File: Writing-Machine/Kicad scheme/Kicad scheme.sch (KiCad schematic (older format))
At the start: 1 part

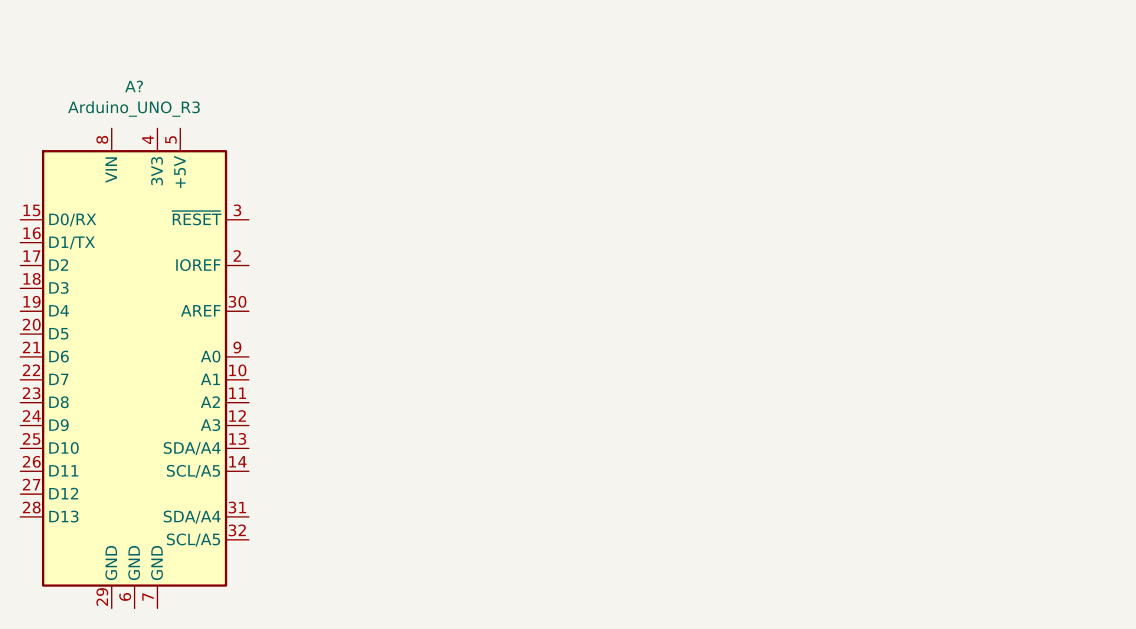
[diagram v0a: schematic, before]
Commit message: Add some work
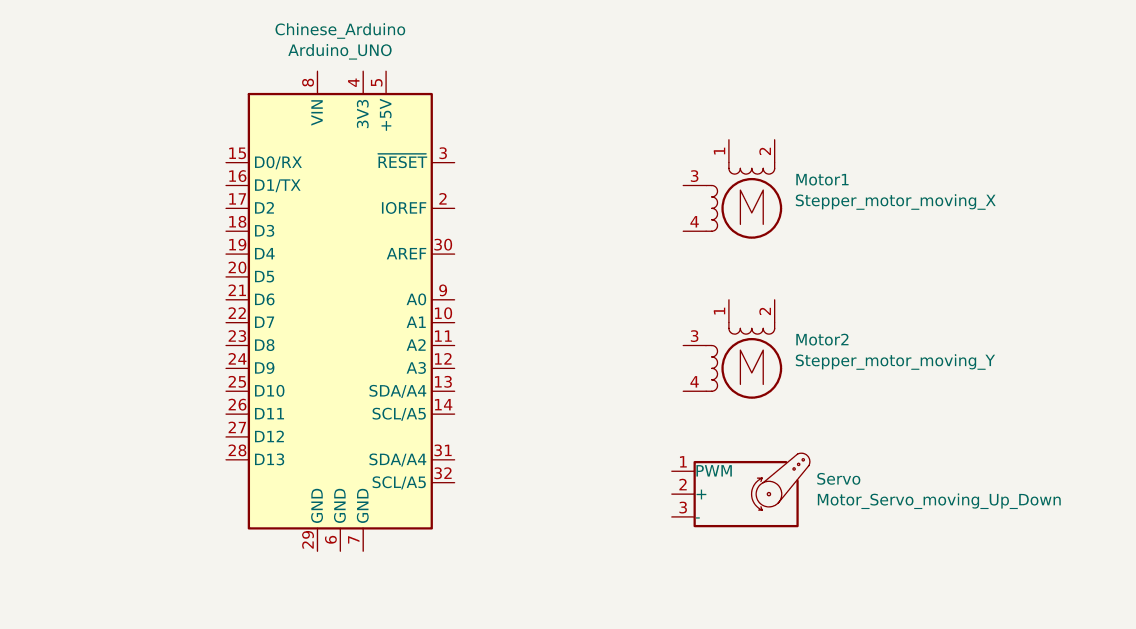
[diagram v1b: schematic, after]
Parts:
- added Motor1: Stepper_motor_moving_X, symbol Motor:Stepper_Motor_bipolar
- added Motor2: Stepper_motor_moving_Y, symbol Motor:Stepper_Motor_bipolar
- added Servo: Motor_Servo_moving_Up_Down, symbol Motor:Motor_Servo
- Chinese_Arduino: renamed from A?; value Arduino_UNO_R3 -> Arduino_UNO
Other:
- moved on the sheet: Chinese_Arduino
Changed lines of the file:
@@
 $EndDescr
 $Comp
-L MCU_Module:Arduino_UNO_R3 A?
+L MCU_Module:Arduino_UNO_R3 Chinese_Arduino
 U 1 1 5FDB88D6
-P 2950 3750
-F 0 "A?" H 2950 4931 50  0000 C CNN
-F 1 "Arduino_UNO_R3" H 2950 4840 50  0000 C CNN
-F 2 "Module:Arduino_UNO_R3" H 2950 3750 50  0001 C CIN
-F 3 "https://www.arduino.cc/en/Main/arduinoBoardUno" H 2950 3750 50  0001 C CNN
-	1    2950 3750
+P 3850 3500
+F 0 "Chinese_Arduino" H 3850 4681 50  0000 C CNN
+F 1 "Arduino_UNO" H 3850 4590 50  0000 C CNN
+F 2 "Module:Arduino_UNO_R3" H 3850 3500 50  0001 C CIN
+F 3 "https://www.arduino.cc/en/Main/arduinoBoardUno" H 3850 3500 50  0001 C CNN
+	1    3850 3500
 	1    0    0    -1
 $EndComp
+$Comp
+L Motor:Stepper_Motor_bipolar Motor1
+U 1 1 5FF2BB4E
+P 5650 3100
+F 0 "Motor1" H 5838 3224 50  0000 L CNN
+F 1 "Stepper_motor_moving_X" H 5838 3133 50  0000 L CNN
+F 2 "" H 5660 3090 50  0001 C CNN
+F 3 "http://www.infineon.com/dgdl/Application-Note-TLE8110EE_driving_UniPolarStepperMotor_V1.1.pdf?fileId=db3a30431be39b97011be5d0aa0a00b0" H 5660 3090 50  0001 C CNN
+	1    5650 3100
+	1    0    0    -1
+$EndComp
+$Comp
+L Motor:Stepper_Motor_bipolar Motor2
+U 1 1 5FF2EFA1
+P 5650 3800
+F 0 "Motor2" H 5838 3924 50  0000 L CNN
+F 1 "Stepper_motor_moving_Y" H 5838 3833 50  0000 L CNN
+F 2 "" H 5660 3790 50  0001 C CNN
+F 3 "http://www.infineon.com/dgdl/Application-Note-TLE8110EE_driving_UniPolarStepperMotor_V1.1.pdf?fileId=db3a30431be39b97011be5d0aa0a00b0" H 5660 3790 50  0001 C CNN
+	1    5650 3800
+	1    0    0    -1
+$EndComp
+$Comp
+L Motor:Motor_Servo Servo
+U 1 1 5FF389CD
+P 5600 4350
+F 0 "Servo" H 5932 4415 50  0000 L CNN
+F 1 "Motor_Servo_moving_Up_Down" H 5932 4324 50  0000 L CNN
+F 2 "" H 5600 4160 50  0001 C CNN
+F 3 "http://forums.parallax.com/uploads/attachments/46831/74481.png" H 5600 4160 50  0001 C CNN
+	1    5600 4350
+	1    0    0    -1
+$EndComp

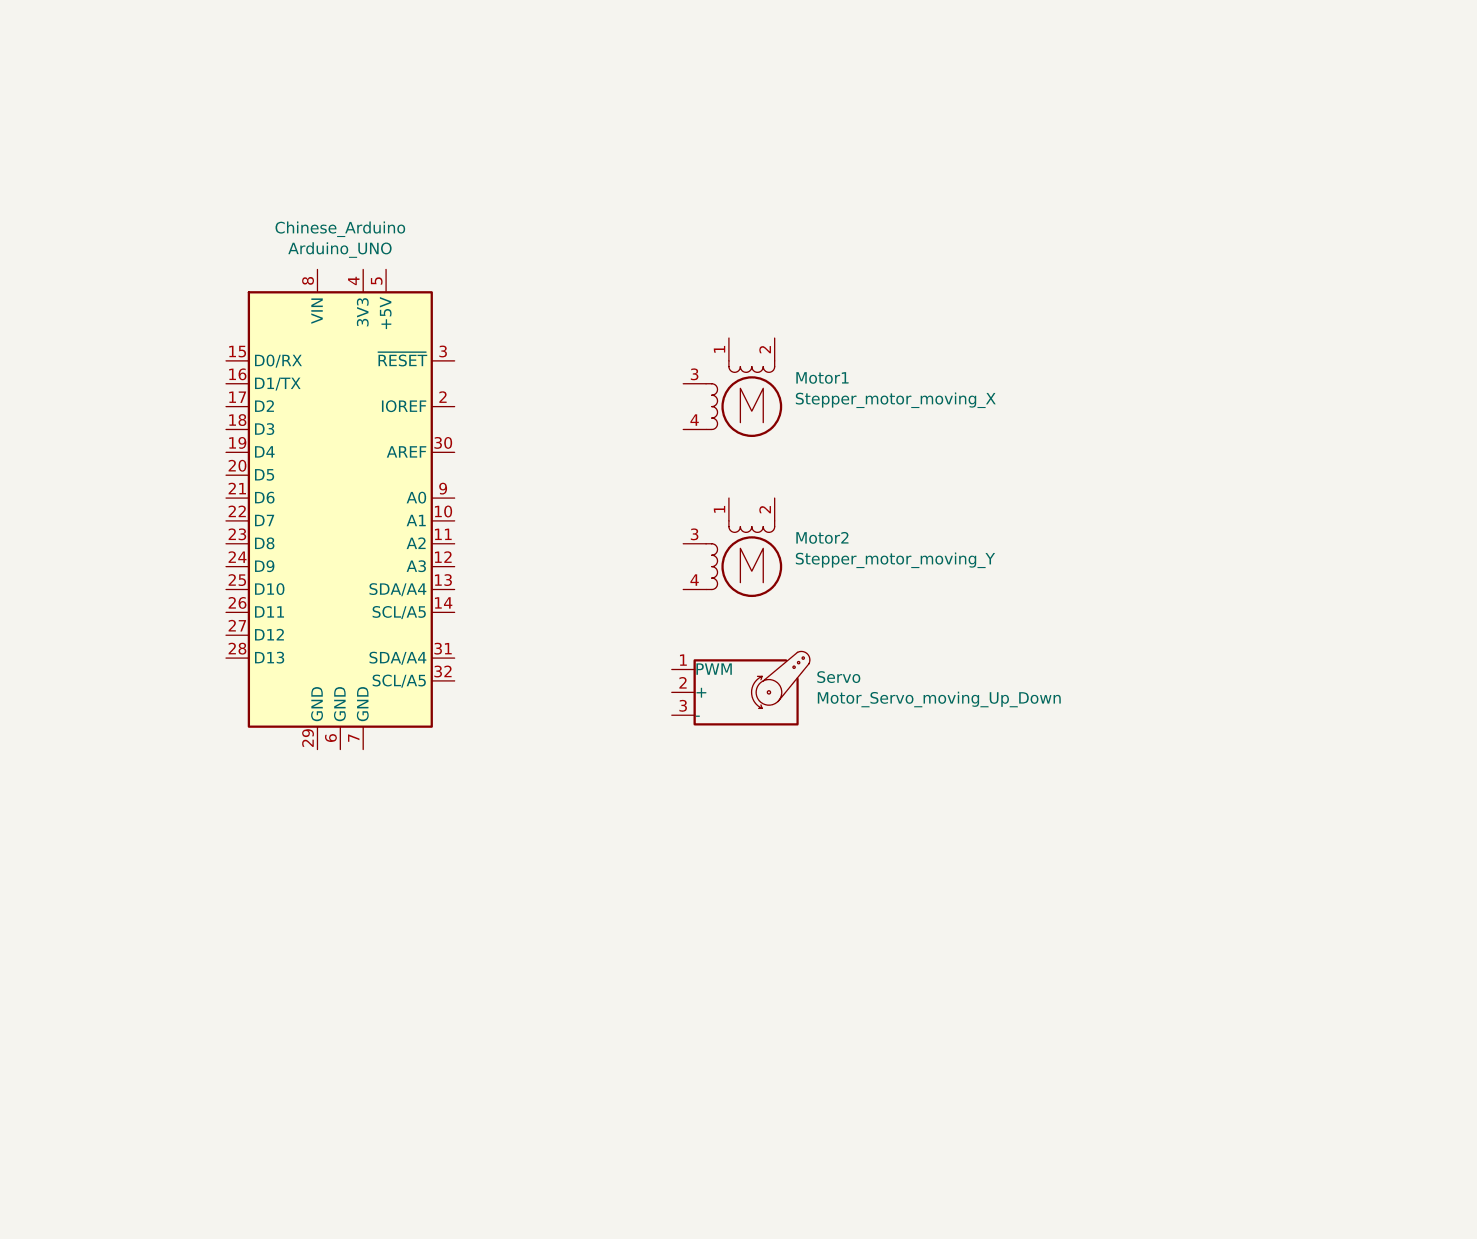
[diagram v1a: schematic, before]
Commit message: Add some night work
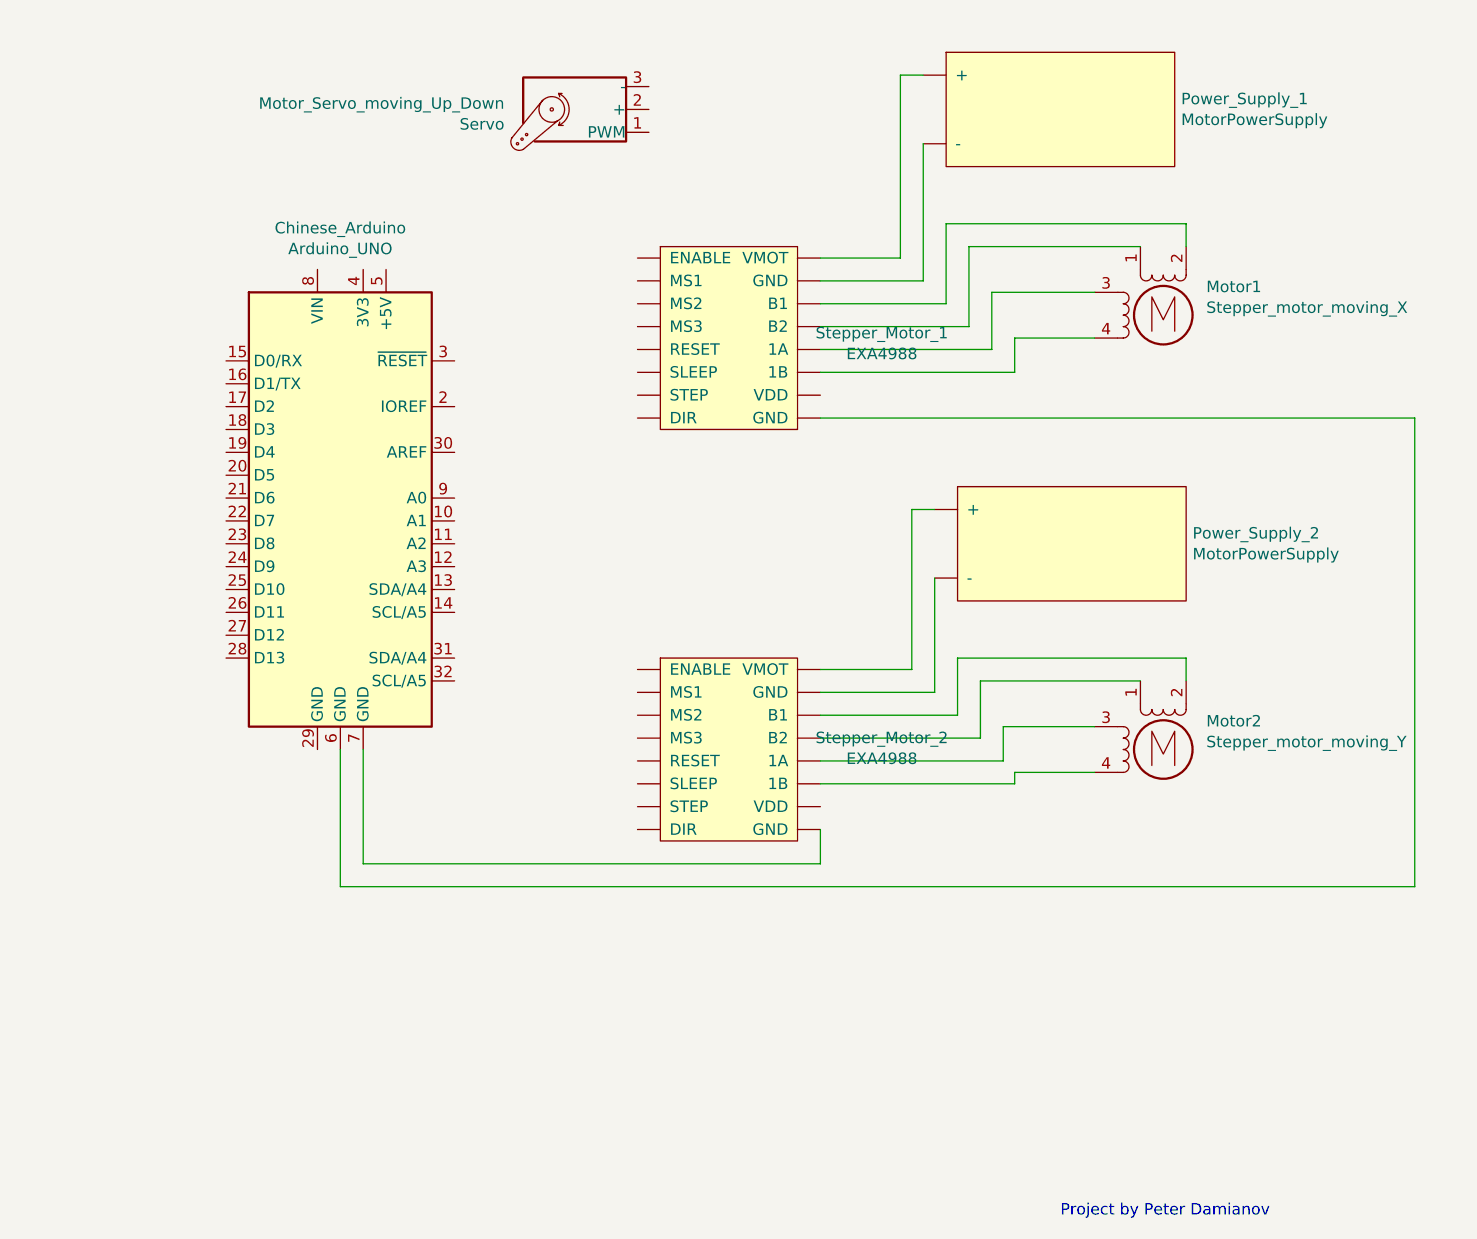
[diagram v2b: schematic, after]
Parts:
- added Power_Supply_1, Power_Supply_2: MotorPowerSupply, symbol Test:MotorPowerSupply
- added Stepper_Motor_1, Stepper_Motor_2: EXA4988, symbol Test:EXA4988
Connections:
- net at Chinese_Arduino.6 (GND): now also Stepper_Motor_1.~ (VMOT)
- net at Chinese_Arduino.7 (GND): now also Stepper_Motor_2.~ (VMOT)
- net at Motor1.1: now also Stepper_Motor_1.~ (VMOT)
- net at Motor1.2 (-): now also Stepper_Motor_1.~ (VMOT)
- net at Motor1.3: now also Stepper_Motor_1.~ (VMOT)
- net at Motor1.4: now also Stepper_Motor_1.~ (VMOT)
- net at Motor2.1: now also Stepper_Motor_2.~ (VMOT)
- net at Motor2.2 (-): now also Stepper_Motor_2.~ (VMOT)
- net at Motor2.3: now also Stepper_Motor_2.~ (VMOT)
- net at Motor2.4: now also Stepper_Motor_2.~ (VMOT)
- new net: Power_Supply_1.~ (-), Stepper_Motor_1.~ (VMOT) (x2)
- new net: Power_Supply_2.~ (-), Stepper_Motor_2.~ (VMOT) (x2)
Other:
- note added: "Project by Peter Damianov"
- moved on the sheet: Motor1, Motor2, Servo
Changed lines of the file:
@@
 L Motor:Stepper_Motor_bipolar Motor1
 U 1 1 5FF2BB4E
-P 5650 3100
-F 0 "Motor1" H 5838 3224 50  0000 L CNN
-F 1 "Stepper_motor_moving_X" H 5838 3133 50  0000 L CNN
-F 2 "" H 5660 3090 50  0001 C CNN
-F 3 "http://www.infineon.com/dgdl/Application-Note-TLE8110EE_driving_UniPolarStepperMotor_V1.1.pdf?fileId=db3a30431be39b97011be5d0aa0a00b0" H 5660 3090 50  0001 C CNN
-	1    5650 3100
+P 7450 2700
+F 0 "Motor1" H 7638 2824 50  0000 L CNN
+F 1 "Stepper_motor_moving_X" H 7638 2733 50  0000 L CNN
+F 2 "" H 7460 2690 50  0001 C CNN
+F 3 "http://www.infineon.com/dgdl/Application-Note-TLE8110EE_driving_UniPolarStepperMotor_V1.1.pdf?fileId=db3a30431be39b97011be5d0aa0a00b0" H 7460 2690 50  0001 C CNN
+	1    7450 2700
 	1    0    0    -1
 $EndComp
@@
 L Motor:Stepper_Motor_bipolar Motor2
 U 1 1 5FF2EFA1
-P 5650 3800
-F 0 "Motor2" H 5838 3924 50  0000 L CNN
-F 1 "Stepper_motor_moving_Y" H 5838 3833 50  0000 L CNN
-F 2 "" H 5660 3790 50  0001 C CNN
-F 3 "http://www.infineon.com/dgdl/Application-Note-TLE8110EE_driving_UniPolarStepperMotor_V1.1.pdf?fileId=db3a30431be39b97011be5d0aa0a00b0" H 5660 3790 50  0001 C CNN
-	1    5650 3800
+P 7450 4600
+F 0 "Motor2" H 7638 4724 50  0000 L CNN
+F 1 "Stepper_motor_moving_Y" H 7638 4633 50  0000 L CNN
+F 2 "" H 7460 4590 50  0001 C CNN
+F 3 "http://www.infineon.com/dgdl/Application-Note-TLE8110EE_driving_UniPolarStepperMotor_V1.1.pdf?fileId=db3a30431be39b97011be5d0aa0a00b0" H 7460 4590 50  0001 C CNN
+	1    7450 4600
 	1    0    0    -1
 $EndComp
@@
 L Motor:Motor_Servo Servo
 U 1 1 5FF389CD
-P 5600 4350
-F 0 "Servo" H 5932 4415 50  0000 L CNN
-F 1 "Motor_Servo_moving_Up_Down" H 5932 4324 50  0000 L CNN
-F 2 "" H 5600 4160 50  0001 C CNN
-F 3 "http://forums.parallax.com/uploads/attachments/46831/74481.png" H 5600 4160 50  0001 C CNN
-	1    5600 4350
+P 4900 1800
+F 0 "Servo" H 5232 1865 50  0000 L CNN
+F 1 "Motor_Servo_moving_Up_Down" H 5232 1774 50  0000 L CNN
+F 2 "" H 4900 1610 50  0001 C CNN
+F 3 "http://forums.parallax.com/uploads/attachments/46831/74481.png" H 4900 1610 50  0001 C CNN
+	1    4900 1800
+	-1   0    0    1
+$EndComp
+$Comp
+L Test:EXA4988 Stepper_Motor_1
+U 1 1 5FFF1309
+P 5550 2800
+F 0 "Stepper_Motor_1" H 6219 2851 50  0000 C TNN
+F 1 "EXA4988" H 6219 2760 50  0000 C TNN
+F 2 "" H 5550 2800 50  0001 C CNN
+F 3 "" H 5550 2800 50  0001 C CNN
+	1    5550 2800
 	1    0    0    -1
 $EndComp
+Wire Wire Line
+	7150 2600 6700 2600
+Wire Wire Line
+	6700 2600 6700 2850
+Wire Wire Line
+	6700 2850 5950 2850
+Wire Wire Line
+	7350 2400 6600 2400
+Wire Wire Line
+	6600 2400 6600 2750
+Wire Wire Line
+	6600 2750 5950 2750
+Wire Wire Line
+	7550 2400 7550 2300
+Wire Wire Line
+	7550 2300 6500 2300
+Wire Wire Line
+	6500 2300 6500 2650
+Wire Wire Line
+	6500 2650 5950 2650
+Wire Wire Line
+	7150 2800 6800 2800
+Wire Wire Line
+	6800 2800 6800 2950
+Wire Wire Line
+	6800 2950 5950 2950
+Wire Wire Line
+	7150 4500 6750 4500
+Wire Wire Line
+	6750 4500 6750 4650
+Wire Wire Line
+	6750 4650 5950 4650
+Wire Wire Line
+	7350 4300 6650 4300
+Wire Wire Line
+	6650 4300 6650 4550
+Wire Wire Line
+	6650 4550 5950 4550
+Wire Wire Line
+	7550 4300 7550 4200
+Wire Wire Line
+	7550 4200 6550 4200
+Wire Wire Line
+	6550 4200 6550 4450
+Wire Wire Line
+	6550 4450 5950 4450
+$Comp
+L Test:EXA4988 Stepper_Motor_2
+U 1 1 5FFF5E11
+P 5550 4600
+F 0 "Stepper_Motor_2" H 6219 4651 50  0000 C CNN
+F 1 "EXA4988" H 6219 4560 50  0000 C CNN
+F 2 "" H 5550 4600 50  0001 C CNN
+F 3 "" H 5550 4600 50  0001 C CNN
+	1    5550 4600
+	1    0    0    -1
+$EndComp
+Wire Wire Line
+	7150 4700 6800 4700
+Wire Wire Line
+	6800 4700 6800 4750
+Wire Wire Line
+	6800 4750 5950 4750
+$Comp
+L Test:MotorPowerSupply Power_Supply_1
+U 1 1 6003464B
+P 7000 1800
+F 0 "Power_Supply_1" H 7528 1846 50  0000 L CNN
+F 1 "MotorPowerSupply" H 7528 1755 50  0000 L CNN
+F 2 "" H 7000 1800 50  0001 C CNN
+F 3 "" H 7000 1800 50  0001 C CNN
+	1    7000 1800
+	1    0    0    -1
+$EndComp
+$Comp
+L Test:MotorPowerSupply Power_Supply_2
+U 1 1 60036794
+P 7050 3700
+F 0 "Power_Supply_2" H 7578 3746 50  0000 L CNN
+F 1 "MotorPowerSupply" H 7578 3655 50  0000 L CNN
+F 2 "" H 7050 3700 50  0001 C CNN
+F 3 "" H 7050 3700 50  0001 C CNN
+	1    7050 3700
+	1    0    0    -1
+$EndComp
+Wire Wire Line
+	6450 3850 6450 4350
+Wire Wire Line
+	6450 4350 5950 4350
+Wire Wire Line
+	6450 3550 6350 3550
+Wire Wire Line
+	6350 3550 6350 4250
+Wire Wire Line
+	6350 4250 5950 4250
+Wire Wire Line
+	6400 1650 6300 1650
+Wire Wire Line
+	6300 1650 6300 2450
+Wire Wire Line
+	6300 2450 5950 2450
+Wire Wire Line
+	6400 1950 6400 2550
+Wire Wire Line
+	6400 2550 5950 2550
+Wire Wire Line
+	3950 5100 5950 5100
+Wire Wire Line
+	5950 5100 5950 4950
+Wire Wire Line
+	3850 4600 3850 5200
+Wire Wire Line
+	3850 5200 8550 5200
+Wire Wire Line
+	8550 3150 5950 3150
+Wire Wire Line
+	8550 3150 8550 5200
+Wire Wire Line
+	3950 4600 3950 5100
+Text Notes 7000 6650 0    50   ~ 0
+Project by Peter Damianov
 $EndSCHEMATC
